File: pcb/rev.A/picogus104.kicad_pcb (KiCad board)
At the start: 4 copper layers, 56 x 87.8 mm, 114 parts, among them J1 USB_C_Receptacle_USB2.0_16P, J10 Conn_01x02_Pin, J11 PC104, J12 PC104_16, J2 DEBUG, J3 IRQDMA_JP, J4 UART_TX, J5 Conn_01x02_Pin, J6 Conn_01x04_Pin, J7 3.5mm TRS, J8 Conn_01x04_Pin, J9 3.5mm TRS, SW1 SW_Push, U1 SN74CB3T3257, U10 PCM5100, U11 W25Q128JVS, U12 RP2040, U13 M62429L, U14 SAM2695, U2 SN74CB3T3257, U3 74AHC14, U4 74LVC00, U5 74LVC00, U6 74LVC2G06DB, U7 SN74CB3T3245, U8 APS6404L-3SQR-SN, U9 AMS1117-3.3_SOT223, Y1 ABLS-12.000MHZ-B4-T, Y2 ABLS-12.000MHZ-B4-T

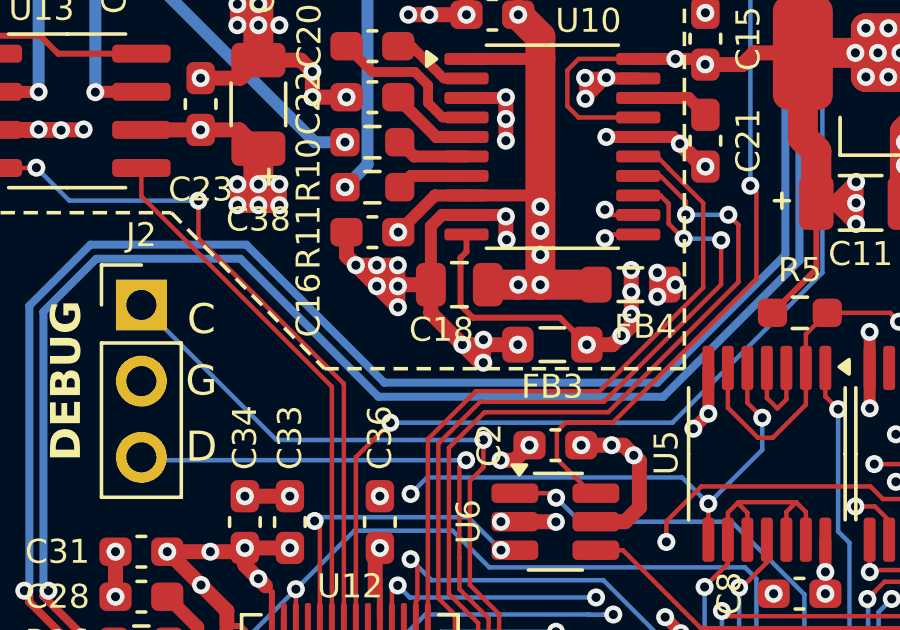
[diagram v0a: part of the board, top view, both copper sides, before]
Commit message: bom fixes
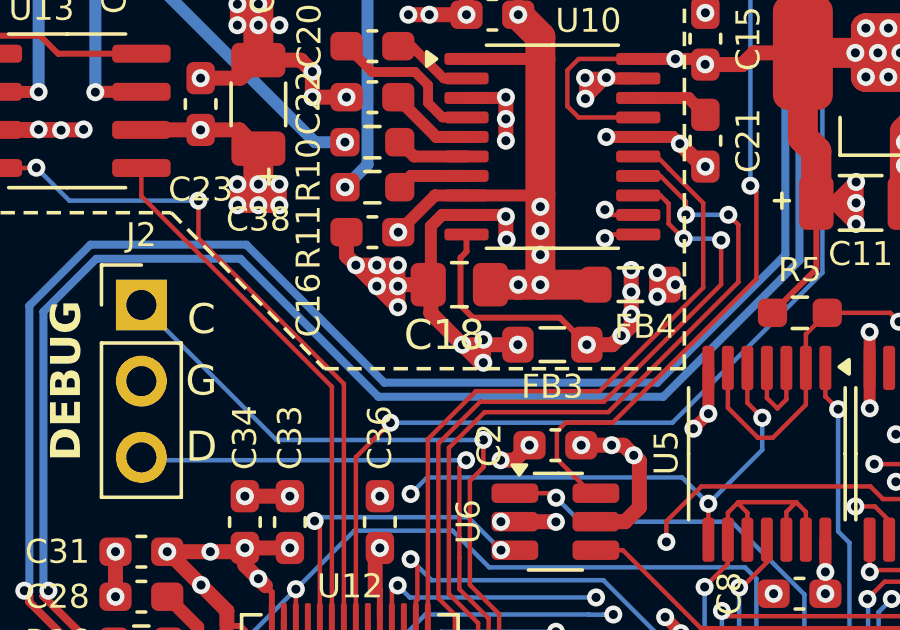
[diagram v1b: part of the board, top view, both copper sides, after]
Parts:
- C12, C13, C47, C49: value 10u -> 10uF
- C18: footprint Capacitor_SMD:C_0805_2012Metric -> Capacitor_SMD:C_0805_2012Metric_Pad1.18x1.45mm_HandSolder
- C50, C51: value 30p -> 30pF
- Y1, Y2: value ABLS-12.000MHZ-B4-T -> 12MHz
